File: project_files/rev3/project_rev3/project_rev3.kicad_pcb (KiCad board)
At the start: 2 copper layers, 86 x 109 mm, 56 parts, among them J1 Barrel_Jack, J2 Conn_01x04, J3 Conn_01x02, J4 Conn_01x02, J5 Conn_01x02, J6 Conn_01x02, J7 Conn_01x02, J8 USB_C_Receptacle_USB2.0_16P, Q1 BSS816NWH6327XTSA1, Q2 S8550, SW1 JS102011SAQN, SW2 PTS810 SJM 250 SMTR LFS, SW3 PTS810 SJM 250 SMTR LFS, U1 HX711, U2 74LS21, U3 AZ1117CH-3.3, U4 MCP6004, U5 ESP32-S3-WROOM-1-N16R8, U6 AZ1117CH-3.3

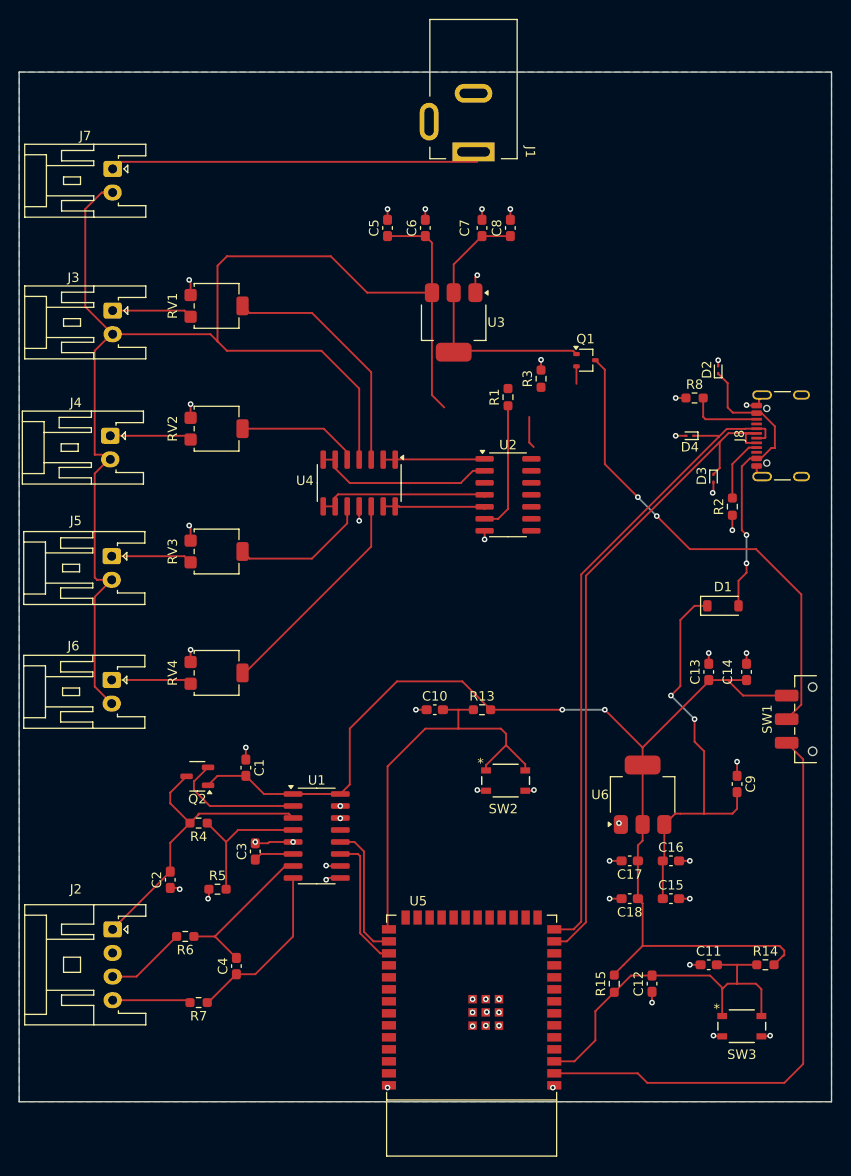
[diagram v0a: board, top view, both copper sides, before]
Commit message: added new project for rev4 and reverted changes for rev3
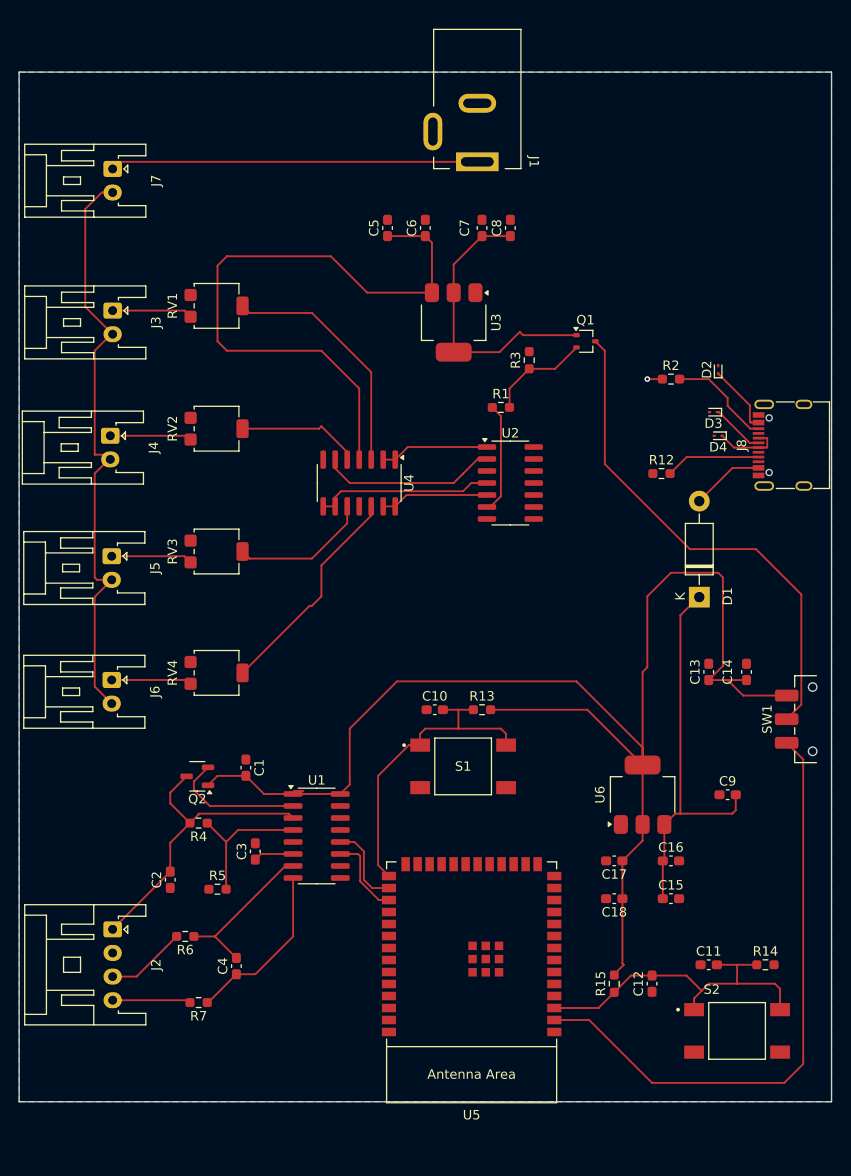
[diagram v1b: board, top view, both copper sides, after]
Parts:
- removed R8: 5.1k, Resistor_SMD:R_0603_1608Metric_Pad0.98x0.95mm_HandSolder
- removed SW2, SW3: PTS810 SJM 250 SMTR LFS, PTS810SJM250SMTR LFS:PTS810_CNK
- added R12: 5.1k, Resistor_SMD:R_0603_1608Metric_Pad0.98x0.95mm_HandSolder, F.Cu at (108.0, 93.0)
- added S1: PTS810SJM250SMTR LFS, TS04-66-95-BK-100-SMT:SW_TS04-66-95-BK-100-SMT, F.Cu at (87.0, 124.0)
- added S2: PTS810SJM250SMTR LFS, TS04-66-95-BK-100-SMT:SW_TS04-66-95-BK-100-SMT, F.Cu at (116.0, 152.0)
- D1: footprint Diode_SMD:D_SOD-123 -> Diode_THT:D_DO-41_SOD81_P10.16mm_Horizontal
- D2, D3, D4: value ESD9B5.0ST5G -> ESD5B5CU
- J8: value USB_C_Receptacle_USB2.0_16P -> USB_C_Receptacle_16P; footprint Connector_USB:USB_C_Receptacle_GCT_USB4105-xx-A_16P_TopMnt_Horizontal -> Connector_USB:USB_C_Receptacle_G-Switch_GT-USB-7010ASV
- moved R2 15.0 mm to (109.0, 83.0), turned to 0 degrees
- moved D3 7.00 mm to (113.5, 86.5), turned to 180 degrees
- moved U5 5.65 mm to (87.9, 143.9)
- moved D4 3.00 mm to (114.0, 89.0)
- moved D1 2.66 mm to (112.0, 106.1), turned to 90 degrees
- moved R3 2.32 mm to (94.0, 81.0)
- moved Q1 2.00 mm to (100.0, 79.0)
- moved C17 1.64 mm to (103.0, 134.0)
- moved C18 1.64 mm to (103.0, 138.0)
- moved C9 1.51 mm to (115.0, 127.0), turned to 0 degrees
- moved R1 1.32 mm to (91.0, 86.0), turned to 0 degrees
- moved U2 1.27 mm to (92.0, 94.0)
- moved J1 1.12 mm to (88.5, 60.0)
- moved J8 1.03 mm to (122.0, 90.0)
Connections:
- net /controller/USB_D+ renamed Net-(D4-A1)
- net /controller/USB_D- renamed Net-(D3-A1)
- net /controller/VBUS renamed Net-(D1-A)
- J8 pad A5: /controller/CC1 -> Net-(J8-CC1)
- J8 pad B5: /controller/CC2 -> Net-(J8-CC2)
- R2 pad 2: /controller/CC1 -> Net-(J8-CC2)
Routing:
- net Net-(D3-A1): track 72.3 -> 5.70 mm
- net Net-(D4-A1): track 70.5 -> 7.15 mm
- net GND: track 54.4 -> 1.59 mm, vias 53 -> 1
- net ESP_3.3V: track 122.4 -> 153.2 mm, vias 2 -> 0
- net +5V_WALL: track 158.4 -> 130.9 mm
- net Net-(D1-A): track 31.0 -> 15.2 mm, vias 2 -> 0
- net GPIO0_BOOT: track 45.2 -> 34.1 mm
- net Net-(J8-CC2): track 0.00 -> 11.0 mm
- net Net-(J8-CC1): track 0.00 -> 10.1 mm
- net Net-(Q1-G): track 2.22 -> 10.9 mm
- net /controller/CC2: track 8.01 -> 0.00 mm
- net /controller/CC1: track 7.38 -> 0.00 mm
- net GPIO_35: track 14.5 -> 8.93 mm
- net GPIO_36: track 14.3 -> 8.73 mm
- net CHIP_PU_EN: track 40.5 -> 37.3 mm
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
